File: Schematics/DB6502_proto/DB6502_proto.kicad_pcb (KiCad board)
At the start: 2 copper layers, 132.1 x 104.1 mm, 51 parts, among them J1 System Bus, J10 AVR-ISP-6, J2 Controls, J3 Debug UART, J4 I/O Bus, J5 USB_B, SW1 Reset, U1 DS1813, U2 65C02S, U3 62256, U4 ATmega644PA-PU, U5 62256, U6 74AC138, U7 28C256, U8 22V10C, U9 FT230XS, Y1 20MHz

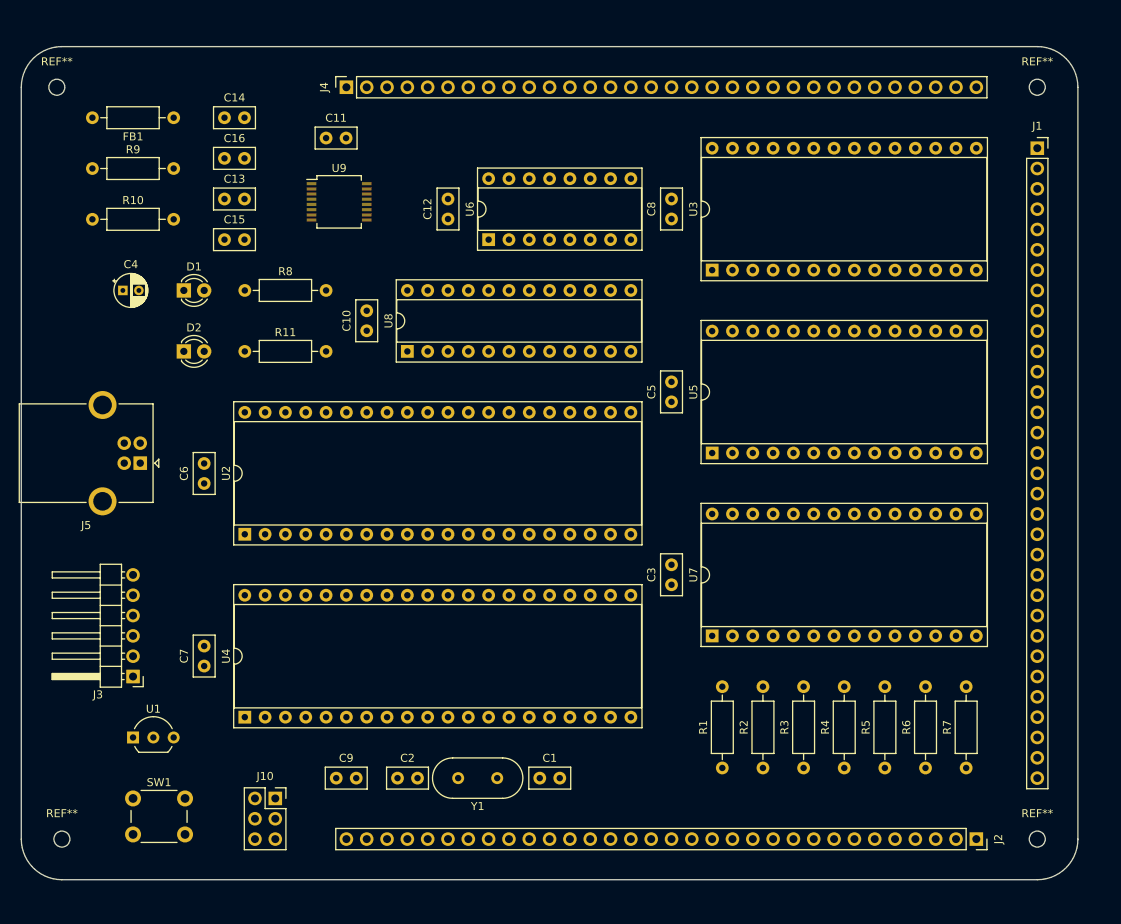
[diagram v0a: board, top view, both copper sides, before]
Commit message: PCB layout RC1
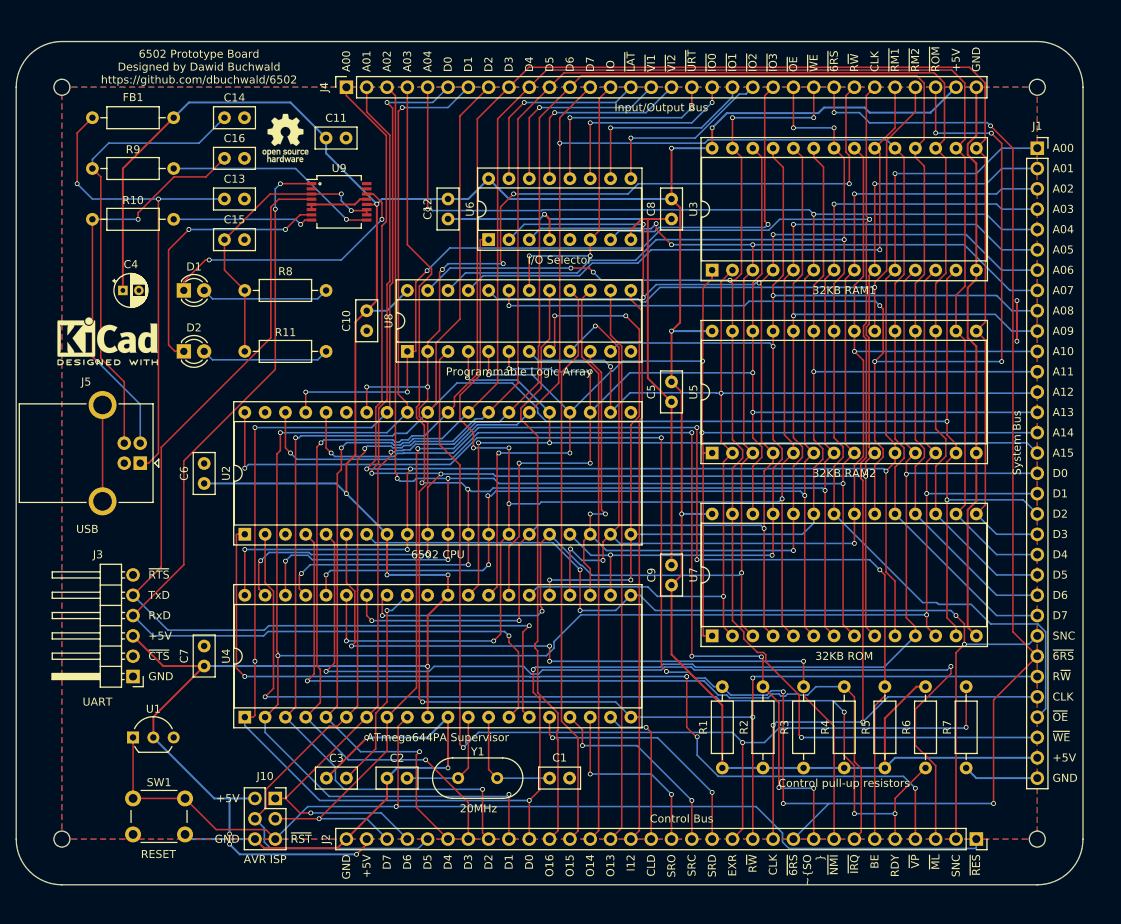
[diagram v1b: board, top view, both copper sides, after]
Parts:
- added REF**: OSHW-Logo_5.7x6mm_SilkScreen, Symbol:OSHW-Logo_5.7x6mm_SilkScreen, F.Cu at (71.1, 24.1)
- added REF**: KiCad-Logo2_5mm_SilkScreen, Symbol:KiCad-Logo2_5mm_SilkScreen, F.Cu at (48.9, 49.5)
- moved C3 49.4 mm to (76.2, 104.1), turned to 0 degrees
- moved C9 48.4 mm to (119.4, 80.0), turned to 90 degrees
- moved C1 3.73 mm to (106.6, 104.1), turned to 180 degrees
- moved C10 2.50 mm to (81.3, 45.7), turned to 270 degrees
- moved C5 2.50 mm to (119.4, 54.6), turned to 270 degrees
- moved C8 2.50 mm to (119.4, 31.8), turned to 270 degrees
- moved C2 1.31 mm to (83.8, 104.1)
- moved REF** 0.63 mm to (43.2, 17.8)
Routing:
- net +5V: track 0.00 -> 473.8 mm, vias 0 -> 12
- net d1: track 0.00 -> 288.2 mm, vias 0 -> 6
- net d0: track 0.00 -> 279.0 mm, vias 0 -> 6
- net ~6502_RES: track 0.00 -> 265.6 mm, vias 0 -> 8
- net d5: track 0.00 -> 261.4 mm, vias 0 -> 1
- net d2: track 0.00 -> 261.3 mm, vias 0 -> 4
- net d3: track 0.00 -> 252.5 mm, vias 0 -> 2
- net d6: track 0.00 -> 248.9 mm, vias 0 -> 2
- net d4: track 0.00 -> 246.8 mm, vias 0 -> 2
- net GND: track 0.00 -> 240.7 mm, vias 0 -> 5
- net d7: track 0.00 -> 239.2 mm, vias 0 -> 3
- net R~W: track 0.00 -> 237.7 mm, vias 0 -> 9
- net a0: track 0.00 -> 230.9 mm, vias 0 -> 6
- net a1: track 0.00 -> 228.6 mm, vias 0 -> 6
- net a2: track 0.00 -> 221.5 mm, vias 0 -> 6
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- added copper zone on B.Cu, net GND
- added copper zone on F.Cu, net GND
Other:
- board size 132.1 x 104.1 mm -> 133.3 x 105.4 mm
- net class Default: clearance 0.2 -> 0.1; trace_width 0.25 -> 0.2; via_dia 0.8 -> 0.6
- net class POWER added: clearance 0.1, trace_width 0.25, via_dia 0.6, via_drill 0.4
- rule trace_clearance: 0.2 -> 0.1
- board text added: "+5V"
- board text added: "20MHz"
- board text added: "32KB RAM1"
- board text added: "32KB RAM2"
- board text added: "32KB ROM"
- board text added: "6502 CPU"
- board text added: "6502 Prototype Board Designed by Dawid Buchwald https://github.com/dbuchwald/6502"
- board text added: "A00"
- board text added: "A01"
- board text added: "A02"
- board text added: "A03"
- board text added: "A04"
- board text added: "A05"
- board text added: "A06"
- board text added: "A07"
- board text added: "A08"
- board text added: "A09"
- board text added: "A10"
- board text added: "A11"
- board text added: "A12"
- board text added: "A13"
- board text added: "A14"
- board text added: "A15"
- board text added: "ATmega644PA Supervisor"
- board text added: "AVR ISP"
- board text added: "BE"
- board text added: "CLD"
- board text added: "CLK"
- board text added: "Control Bus"
- board text added: "Control pull-up resistors"
- board text added: "D0"
- board text added: "D1"
- board text added: "D2"
- board text added: "D3"
- board text added: "D4"
- board text added: "D5"
- board text added: "D6"
- board text added: "D7"
- board text added: "EXR"
- board text added: "GND"
- board text added: "I/O Selector"
- board text added: "I12"
- board text added: "IO"
- board text added: "Input/Output Bus"
- board text added: "O13"
- board text added: "O14"
- board text added: "O15"
- board text added: "O16"
- board text added: "Programmable Logic Array"
- board text added: "RDY"
- board text added: "RESET"
- board text added: "RxD"
- board text added: "R~W"
- board text added: "SNC"
- board text added: "SRC"
- board text added: "SRD"
- board text added: "SRO"
- board text added: "System Bus"
- board text added: "TxD"
- board text added: "UART"
- board text added: "USB"
- board text added: "~6RS"
- board text added: "~CTS"
- board text added: "~IO0"
- board text added: "~IO1"
- board text added: "~IO2"
- board text added: "~IO3"
- board text added: "~IRQ"
- board text added: "~LAT"
- board text added: "~ML"
- board text added: "~NMI"
- board text added: "~OE"
- board text added: "~RES"
- board text added: "~RM1"
- board text added: "~RM2"
- board text added: "~ROM"
- board text added: "~RST"
- board text added: "~RTS"
- board text added: "~SO"
- board text added: "~URT"
- board text added: "~VI1"
- board text added: "~VI2"
- board text added: "~VP"
- board text added: "~WE"
